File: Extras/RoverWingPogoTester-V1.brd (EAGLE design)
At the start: 81.3 x 81.3 mm, 10 parts

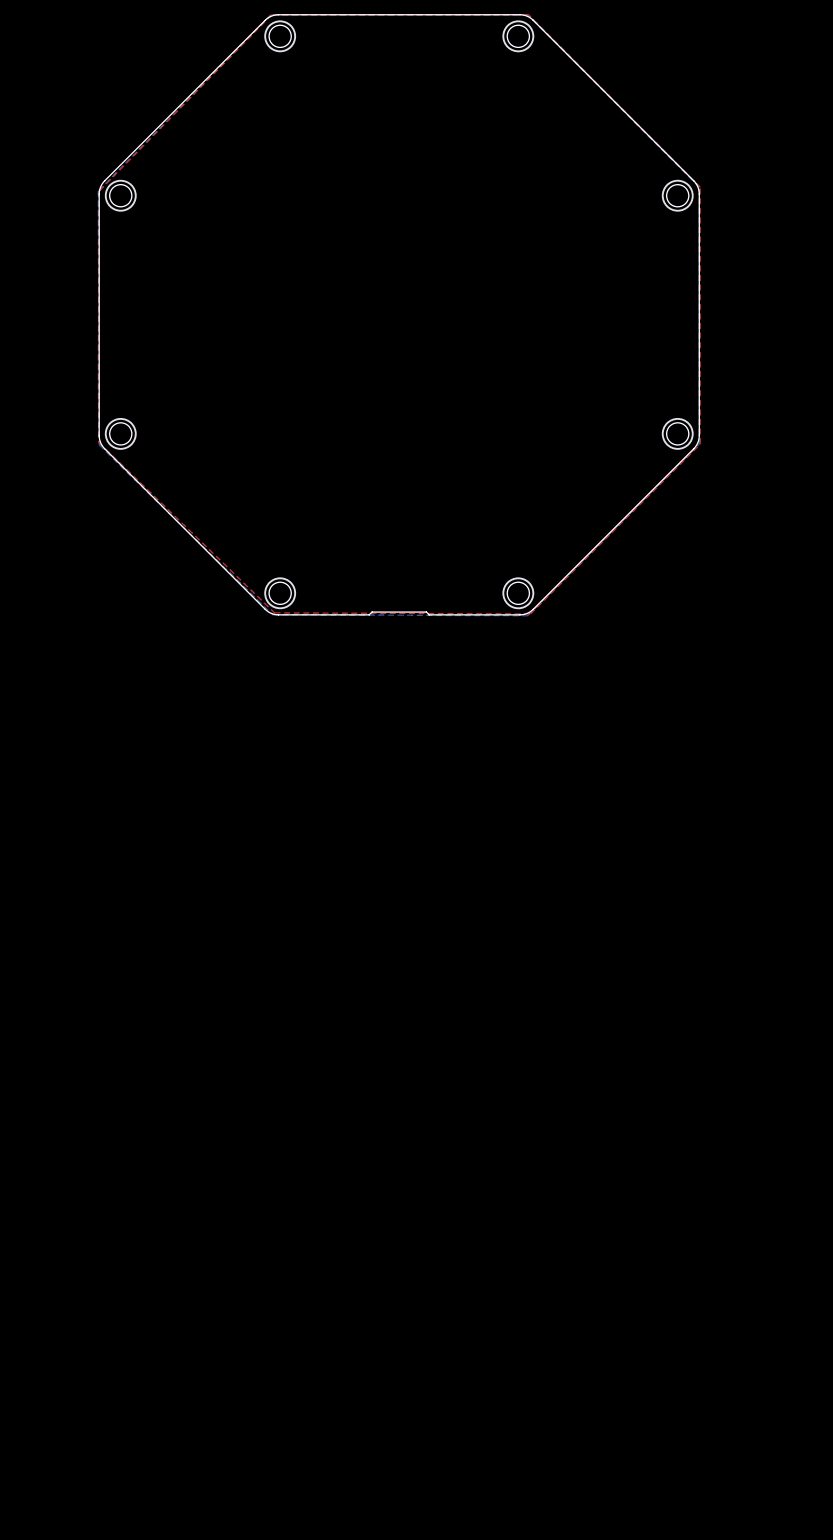
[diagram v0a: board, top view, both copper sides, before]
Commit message: Pogo Tester design finished
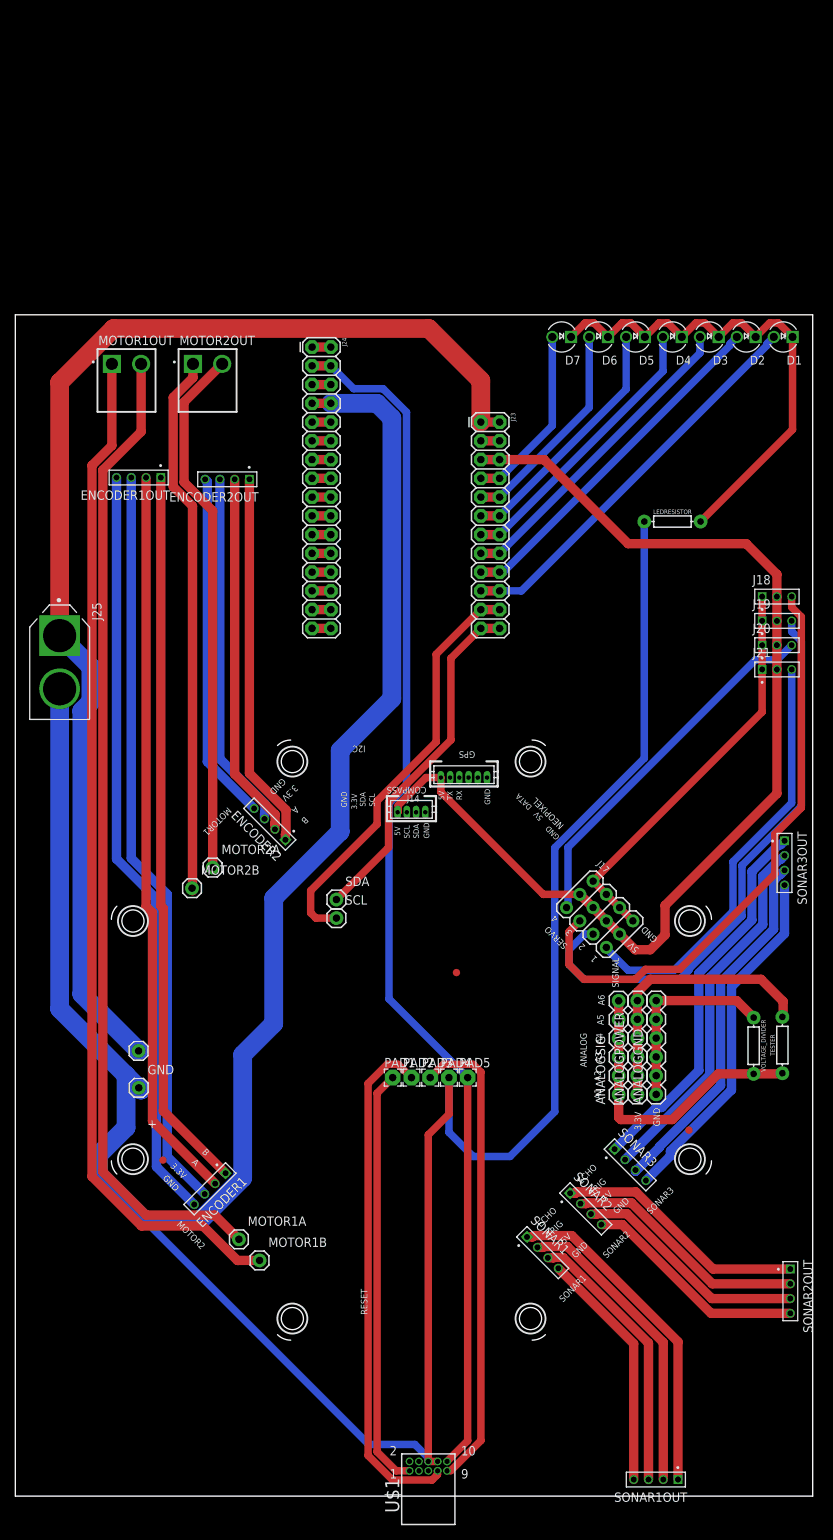
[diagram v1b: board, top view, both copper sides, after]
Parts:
- removed FRAME1, FRAME2: FRAME-LETTERNO_PACKAGE, SparkFun-Aesthetics:DUMMY
- added ANALOGGND, ANALOGPOWER, ANALOGSIG: (no value), SparkFun:1X06
- added D1, D2, D3, D4, D5, D6, D7: LTL-1CHG, LED:RADIAL_3MM
- added ENCODER1, ENCODER1OUT, ENCODER2, ENCODER2OUT, SONAR1, SONAR1OUT, SONAR2, SONAR2OUT, SONAR3, SONAR3OUT: 62000411121, Headers:62000411121
- added FRAME3: FRAME-LETTERNO_PACKAGE, RoverWing-V1.5:DUMMY
- added GND, MOTOR1A, MOTOR1B, MOTOR2A, MOTOR2B, SCL, SDA, VIN: M01PTH, SparkFun:1X01
- added J14: DF13-4P-1.25DSA, RoverWing-V1.5:DF13-4P-1.25DSA
- added J15: DF13-6P-1.25DSA, RoverWing-V1.5:DF13-6P-1.25DSA
- added J17: HEADER-3X04, RoverWing-V1.5:3X04
- added J18, J19, J20, J21: 62000311121, Headers:62000311121
- added J23: HEADER-2X12, RoverWing-V1.5:2X12
- added J24: HEADER-2X16, RoverWing-V1.5:2X16
- added J25: XT60-M, XT60-M:AMASS_XT60-M
- added LEDRESISTOR, TESTER, VOLTAGE_DIVIDER: 10k, SparkFun-Resistors:AXIAL-0.3
- added MOTOR1OUT, MOTOR2OUT: B2P-VH(LF)(SN), Connectors:HDR-02
- added PAD1, PAD2, PAD3, PAD4, PAD5: (no value), wirepad:2,15/1,0
- added U$1: SAMTEC-FTSH-105-01-X-D-RAJ, SAMTEC-FTSH-105-01-X-D-RA:SAMTEC-FTSH-105-01-X-D-RA
- added U$11, U$13, U$17: FIDUCIAL, RoverWing-V1.5:FIDUCIAL_1MM
- U$14, U$15, U$24, U$25, U$26, U$27, U$3, U$4: device CrickitCopy:MOUNTINGHOLE_3.0_NPH -> RoverWing-V1.5:MOUNTINGHOLE_3.0_NPH
- moved U$15 98.2 mm to (-36.1, -82.1)
- moved U$25 98.2 mm to (39.4, -82.1)
- moved U$14 98.2 mm to (-36.1, -114.4)
- moved U$24 98.2 mm to (39.4, -114.4)
- moved U$26 98.2 mm to (-14.5, -60.5)
- moved U$27 98.2 mm to (17.8, -60.5)
- moved U$3 98.2 mm to (-14.5, -136.0)
- moved U$4 98.2 mm to (17.8, -136.0)
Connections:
- new net !RESET1: J24.1, J24.2
- new net 11: ENCODER1.1, ENCODER1OUT.1
- new net 12: ENCODER1.2, ENCODER1OUT.2
- new net 13: ENCODER1.3, ENCODER1OUT.3
- new net 14: ENCODER1.4, ENCODER1OUT.4
- new net 21: ENCODER2.1, ENCODER2OUT.1
- new net 22: ENCODER2.2, ENCODER2OUT.2
- new net 23: ENCODER2.3, ENCODER2OUT.3
- new net 24: ENCODER2.4, ENCODER2OUT.4
- new net 3.3V: J24.3, J24.4, PAD5.1, U$1.10
- new net 5V: J14.P$1, J15.P$1, J17.11, J17.2, J17.5, J17.8, J18.2, J19.2, J20.2, J21.2, J23.5, J23.6
- new net D10: D6.A, J23.10, J23.9
- new net D11: D7.A, J23.7, J23.8
- new net D5: D1.A, J23.19, J23.20
- new net D6: D2.A, J23.17, J23.18
- new net D7: D3.A, J23.15, J23.16
- new net D8: D4.A, J23.13, J23.14
- new net D9: D5.A, J23.11, J23.12
- new net GND: GND.1, J14.P$4, J15.P$6, J17.12, J17.3, J17.6, J17.9, J18.1, J19.1, J20.1, J21.1, J24.7, J24.8, J25.2, LEDRESISTOR.P$1, PAD4.1, U$1.6, U$1.8
- new net LEDGND: D1.C, D2.C, D3.C, D4.C, D5.C, D6.C, D7.C, LEDRESISTOR.P$2
- new net N$1: MOTOR1A.1, MOTOR1OUT.2
- new net N$10: SONAR2.4, SONAR2OUT.4
- new net N$11: SONAR2.3, SONAR2OUT.3
- new net N$12: SONAR2.2, SONAR2OUT.2
- new net N$13: SONAR2.1, SONAR2OUT.1
- new net N$14: SONAR3.4, SONAR3OUT.4
- new net N$15: SONAR3.3, SONAR3OUT.3
- new net N$16: SONAR3.2, SONAR3OUT.2
- new net N$17: SONAR3.1, SONAR3OUT.1
- new net N$18: ANALOGSIG.1, ANALOGSIG.2, ANALOGSIG.3, ANALOGSIG.4, ANALOGSIG.5, ANALOGSIG.6, TESTER.P$1, VOLTAGE_DIVIDER.P$2
- new net N$2: MOTOR1B.1, MOTOR1OUT.1
- new net N$23: ANALOGGND.1, ANALOGGND.2, ANALOGGND.3, ANALOGGND.4, ANALOGGND.5, ANALOGGND.6, VOLTAGE_DIVIDER.P$1
- new net N$24: J23.3, J23.4
- new net N$26: J15.P$4
- new net N$27: J15.P$5
- new net N$3: MOTOR2A.1, MOTOR2OUT.2
- new net N$34: J24.5, J24.6
- new net N$35: J24.10, J24.9
- new net N$36: J24.11, J24.12
- new net N$37: J24.13, J24.14
- new net N$38: J24.15, J24.16
- new net N$39: J24.17, J24.18
- new net N$4: MOTOR2B.1, MOTOR2OUT.1
- new net N$47: J24.19, J24.20
- new net N$5: SONAR1.4, SONAR1OUT.4
- new net N$6: SONAR1.3, SONAR1OUT.3
- new net N$60: J24.21, J24.22
- new net N$61: J24.23, J24.24
- new net N$62: J24.25, J24.26
- new net N$63: J24.27, J24.28
- new net N$64: J24.29, J24.30
- new net N$65: J24.31, J24.32
- new net N$7: SONAR1.2, SONAR1OUT.2
- new net N$8: ANALOGPOWER.1, ANALOGPOWER.2, ANALOGPOWER.3, ANALOGPOWER.4, ANALOGPOWER.5, ANALOGPOWER.6, TESTER.P$2
- new net N$9: SONAR1.1, SONAR1OUT.1
- new net RESET: PAD1.1, U$1.1
- new net RX: J15.P$3
- new net SCL1: J23.21, J23.22, SCL.1
- new net SCL2: J14.P$2
- new net SDA1: J23.23, J23.24, SDA.1
- new net SDA2: J14.P$3
- new net SERVO1: J17.1, J20.3
- new net SERVO2: J17.4, J18.3
- new net SERVO3: J17.7, J19.3
- new net SERVO4: J17.10, J21.3
- new net SWCLK: PAD2.1, U$1.7
- new net SWDIO: PAD3.1, U$1.9
- new net TX: J15.P$2
- new net VIN: J23.1, J23.2, J25.1, VIN.1
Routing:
- net GND: track 0.00 -> 494.9 mm
- net VIN: track 0.00 -> 167.1 mm
- net 3.3V: track 0.00 -> 164.1 mm
- net 5V: track 0.00 -> 152.0 mm
- net N$2: track 0.00 -> 138.6 mm
- net N$1: track 0.00 -> 133.8 mm
- net 14: track 0.00 -> 102.8 mm
- net 13: track 0.00 -> 101.2 mm
- net 12: track 0.00 -> 99.5 mm
- net 11: track 0.00 -> 97.9 mm
- net SERVO2: track 0.00 -> 80.7 mm
- net SERVO3: track 0.00 -> 77.9 mm
- net N$4: track 0.00 -> 73.9 mm
- net N$3: track 0.00 -> 72.0 mm
- net SWCLK: track 0.00 -> 69.7 mm
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- removed copper zone on layer 1, net GND
- removed copper zone on layer 16, net GND
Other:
- board size 81.3 x 81.3 mm -> 108 x 160 mm
- board text added: "+"
- board text added: "1"
- board text added: "2"
- board text added: "3"
- board text added: "3.3V"
- board text added: "4"
- board text added: "5V"
- board text added: "A"
- board text added: "A1"
- board text added: "A2"
- board text added: "A3"
- board text added: "A4"
- board text added: "A5"
- board text added: "A6"
- board text added: "ANALOG"
- board text added: "B"
- board text added: "COMPASS"
- board text added: "DATA"
- board text added: "ECHO"
- board text added: "GND"
- board text added: "GPS"
- board text added: "I2C"
- board text added: "MOTOR1"
- board text added: "MOTOR2"
- board text added: "NEOPIXEL"
- board text added: "RESET"
- board text added: "RX"
- board text added: "RoverWing V2.2 D. Bershadsky, A. Kirillov github.com/roverwing"
- board text added: "SCL"
- board text added: "SDA"
- board text added: "SERVO"
- board text added: "SIGNAL"
- board text added: "SONAR1"
- board text added: "SONAR2"
- board text added: "SONAR3"
- board text added: "TRIG"
- board text added: "TX"
